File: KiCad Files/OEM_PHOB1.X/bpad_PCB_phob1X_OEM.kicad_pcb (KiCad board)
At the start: 2 copper layers, 31.6 x 51.6 mm, 24 parts, among them J1 Conn_01x04, SW1 C_left, SW2 C_up, SW3 C_down, SW4 C_right

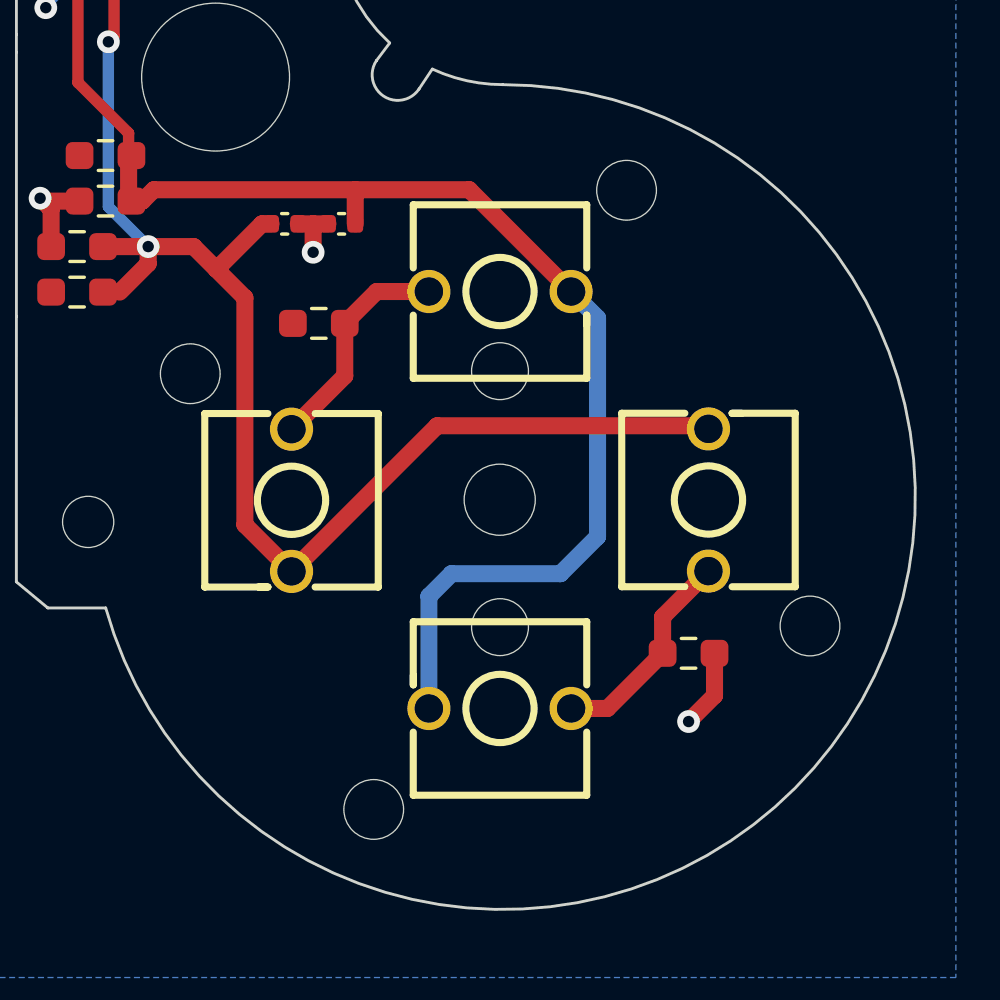
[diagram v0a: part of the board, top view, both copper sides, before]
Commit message: gerbers for ordering (needs to be cleaned)
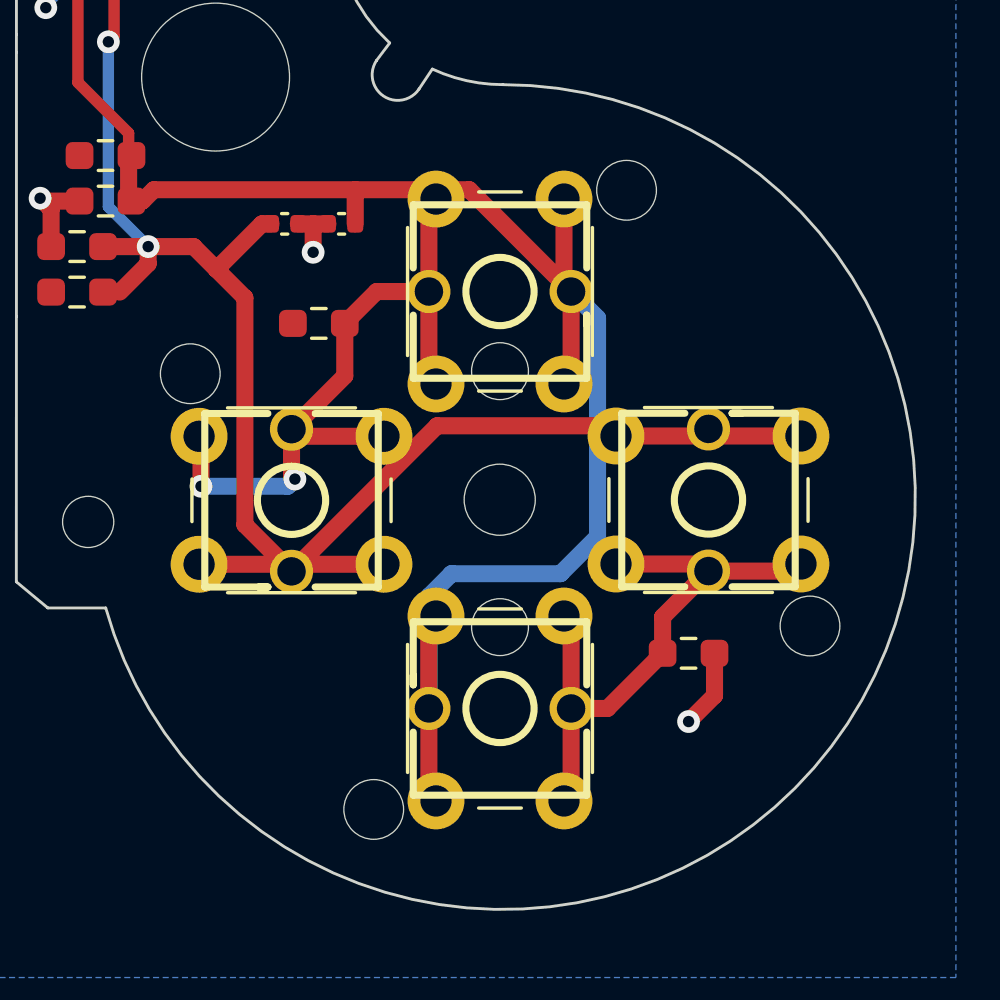
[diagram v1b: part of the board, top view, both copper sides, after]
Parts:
- added REF**: SW_PUSH_6mm, Button_Switch_THT:SW_PUSH_6mm, F.Cu at (134.1, 106.1)
- added REF**: SW_PUSH_6mm, Button_Switch_THT:SW_PUSH_6mm, F.Cu at (138.6, 114.3)
- added REF**: SW_PUSH_6mm, Button_Switch_THT:SW_PUSH_6mm, F.Cu at (146.9, 112.5)
- added REF**: SW_PUSH_6mm, Button_Switch_THT:SW_PUSH_6mm, F.Cu at (125.8, 108.0)
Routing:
- net Net-(R2-Pad1): track 7.92 -> 25.0 mm, vias 0 -> 2
- net /C_x: track 65.3 -> 78.7 mm
- net Net-(R1-Pad1): track 7.58 -> 21.0 mm
- net /C_y: track 63.4 -> 73.9 mm
